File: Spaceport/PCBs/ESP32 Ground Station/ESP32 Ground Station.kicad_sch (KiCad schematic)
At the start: 49 parts, among them J1 Micro_SD_Card_Det1, J2 BAT, J3 USB_C_Receptacle_USB2.0_16P, J4 SMA, J7 Conn_01x10, J8 Conn_01x10, SW1 SW_SPST, U1 ESP32-S3-MINI-1, U2 LBAA0XV2GT-001, U3 XC6220B331MR, U4 USBLC6-2P6, U5 TPS22917DBV, U6 BQ25185DLHR

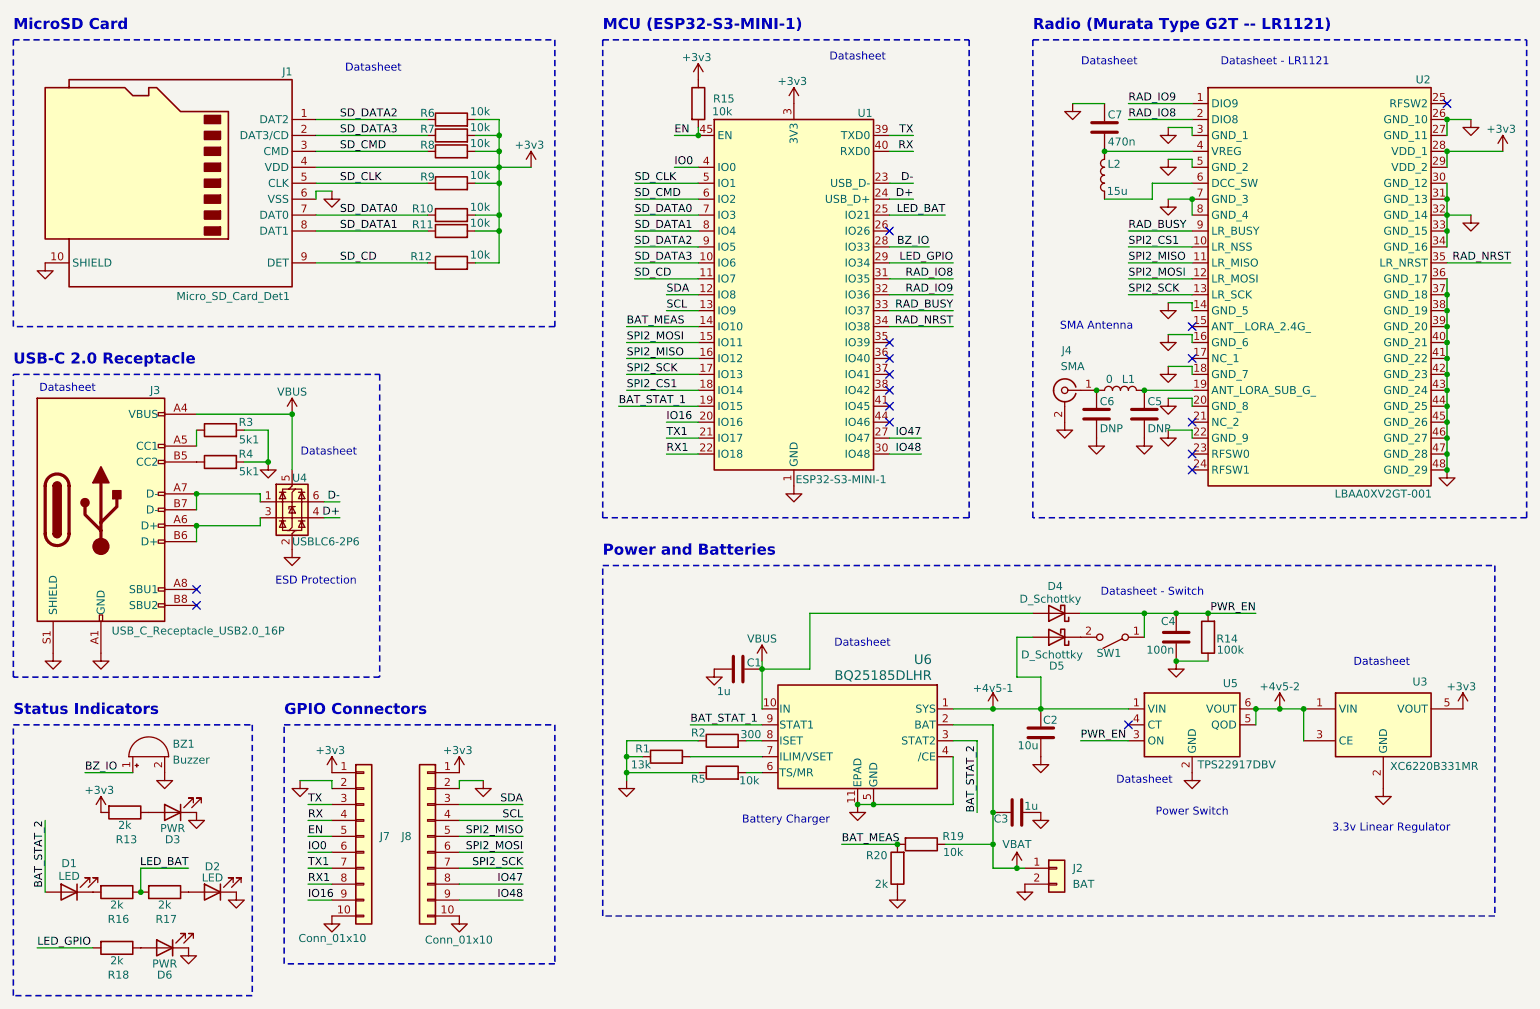
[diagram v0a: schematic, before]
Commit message: add decoupling caps
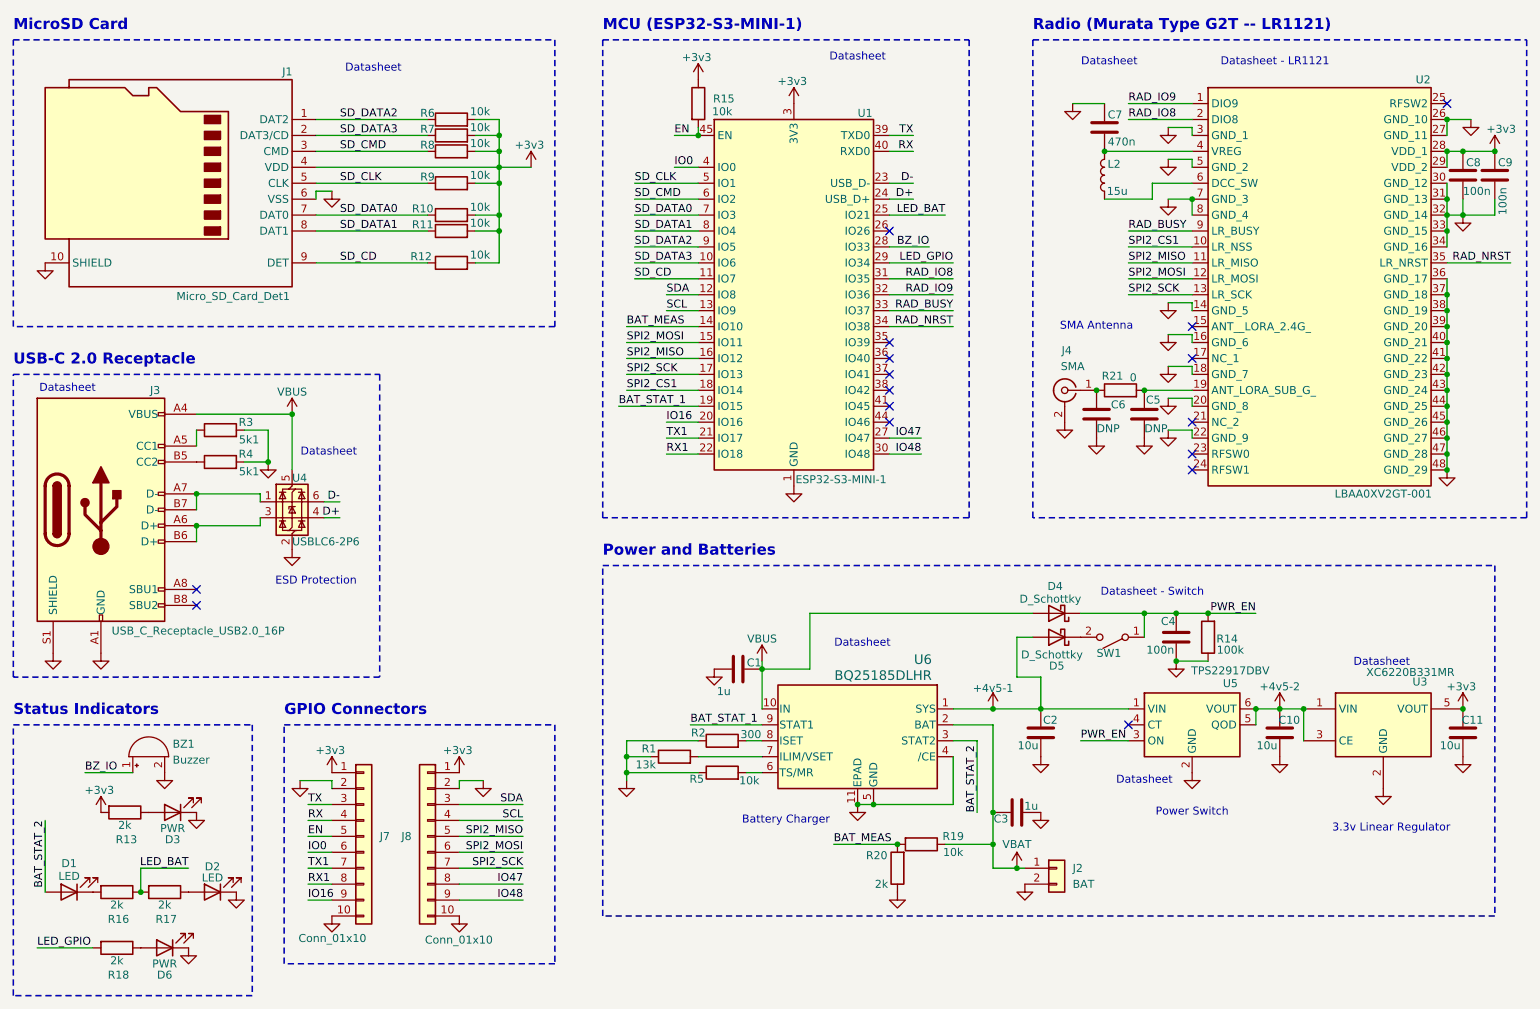
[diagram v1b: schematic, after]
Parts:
- removed L1: 0, Inductor_SMD:L_0603_1608Metric, symbol Device:L
- added C10, C11: 10u, Capacitor_SMD:C_0603_1608Metric, symbol Device:C
- added C8, C9: 100n, Capacitor_SMD:C_0603_1608Metric, symbol Device:C
- added R21: 0, Resistor_SMD:R_0603_1608Metric, symbol Device:R
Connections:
- net +3v3: now also C11.2, C8.1, C9.1
- net +4v5-2: now also C10.2
- net GND: now also C10.1, C11.1, C8.2, C9.2
- net at C6.1, J4.1 (In): now also R21.1
- net at C5.1, U2.19 (ANT_LORA_SUB_G_): now also R21.2
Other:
- moved on the sheet: R1
